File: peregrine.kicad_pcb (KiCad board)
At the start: 4 copper layers, 113.2 x 20.4 mm, 52 parts, among them J1 Barrel_Jack, J2 Ext., J3 Ext., J4 50Ω, SW1 SW_SPDT, SW2 SW_SPDT, U1 MIC5365-3.3YD5, U2 MIC5365-3.3YD5, U3 4020, U4 TS5A3159ADBVR, U5 74AUC1G86, U6 74AUC2G34, X1 ASV-16MHz

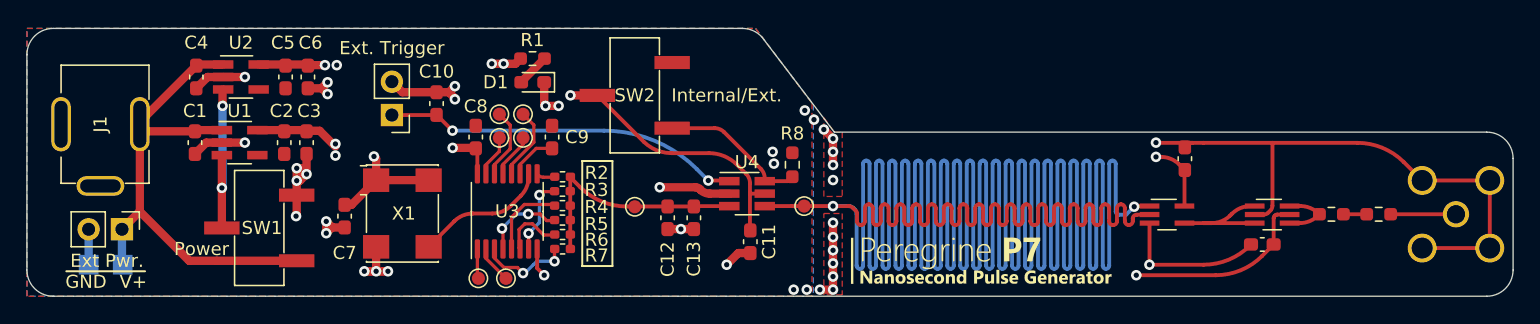
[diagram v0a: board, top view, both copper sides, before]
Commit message: this concerns me
i feel like this is not going to be pretty. might need to simulate more
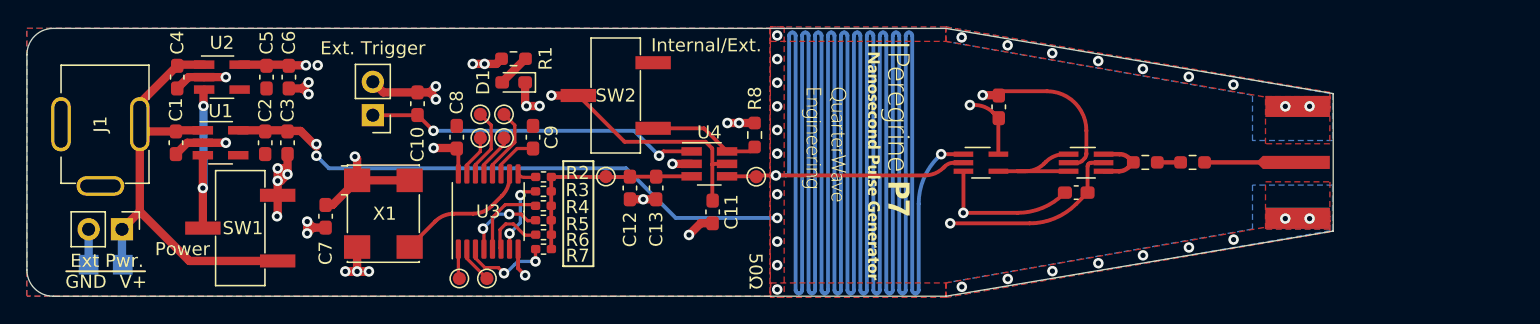
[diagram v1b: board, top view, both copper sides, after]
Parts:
- removed the G*** at (161.8, 104.7)
- added G***: LOGO, QuarterWave:logoWithText12mmPartialMask, F.Cu at (153.7, 101.7)
- J4: footprint SMA_RightAngle:SMA-RightAngle -> CONSMA020:LINX_CONSMA020.062-G
- moved R10 14.7 mm to (181.8, 104.6)
- moved R9 14.7 mm to (178.2, 104.6)
- moved C14 14.7 mm to (167.0, 100.4)
- moved C15 14.7 mm to (172.9, 106.9)
- moved U5 14.7 mm to (165.7, 104.6)
- moved U6 14.7 mm to (173.7, 104.6)
- moved G*** 10.4 mm to (158.6, 104.6), turned to -90 degrees
- moved J4 10.4 mm to (192.2, 104.6), turned to 90 degrees
- moved TP3 4.28 mm to (148.6, 105.7)
- moved C12 3.66 mm to (138.9, 106.6)
- moved C13 3.66 mm to (140.9, 106.6)
- moved C11 3.66 mm to (145.2, 108.4)
- moved R8 3.66 mm to (148.4, 102.5)
- moved U4 3.66 mm to (145.0, 104.7)
- moved TP4 3.18 mm to (137.1, 105.7)
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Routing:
- net GND: track 119.1 -> 72.2 mm, vias 40 -> 53
- net VCC: track 127.6 -> 134.0 mm
- net Trig: track 420.2 -> 426.0 mm
- net +VDC: track 39.6 -> 36.1 mm
- net Net-(R8-Pad1): track 11.2 -> 8.60 mm
- net FTrig: track 18.5 -> 16.4 mm
- net Net-(J4-Pad1): track 4.97 -> 6.74 mm
- net +3V3: track 75.8 -> 74.1 mm
- net Net-(C10-Pad1): track 27.3 -> 25.8 mm
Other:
- board size 113.2 x 20.4 mm -> 99.5 x 20.4 mm

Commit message: redesign
why yes i redesigned half of the entire board
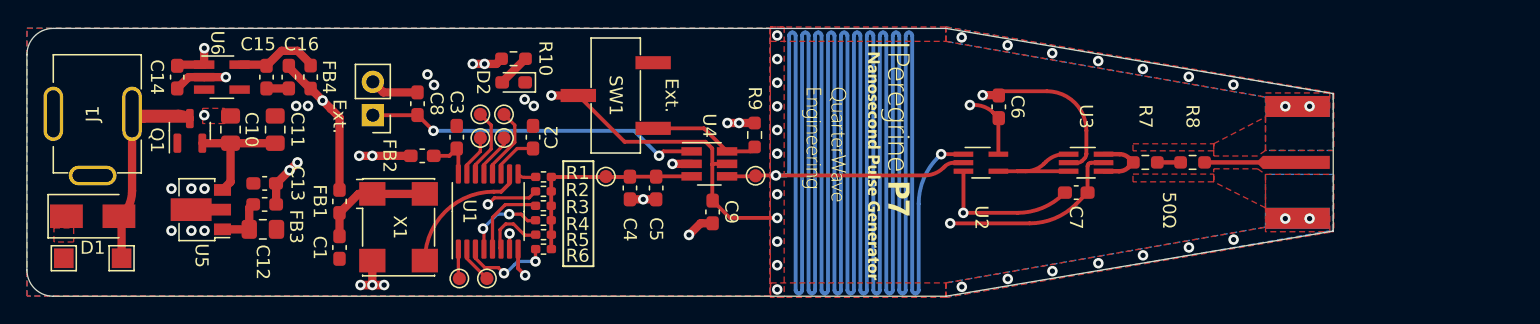
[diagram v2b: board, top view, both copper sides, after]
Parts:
- removed the C1 at (104.3, 103.1)
- removed the C2 at (111.2, 103.1)
- removed the J2 at (100.2, 109.7)
- removed the SW1 at (109.2, 109.6)
- removed the TP1 at (100.3, 112.4)
- removed the TP2 at (97.7, 112.4)
- removed the U1 at (107.8, 103.1)
- added C10: 10μF, Capacitor_SMD:C_0805_2012Metric_Pad1.18x1.45mm_HandSolder, F.Cu at (108.5, 102.1)
- added C11: 330nF, Capacitor_SMD:C_0805_2012Metric_Pad1.18x1.45mm_HandSolder, F.Cu at (111.9, 102.1)
- added C12: 10μF, Capacitor_SMD:C_0805_2012Metric_Pad1.18x1.45mm_HandSolder, F.Cu at (111.0, 109.7)
- added D1: SMAJ30A, Diode_SMD:D_SMA, F.Cu at (98.0, 108.7)
- added FB1: FerriteBead_Small, Inductor_SMD:L_0603_1608Metric_Pad1.05x0.95mm_HandSolder, F.Cu at (116.8, 107.6)
- added FB2: FerriteBead_Small, Inductor_SMD:L_0603_1608Metric_Pad1.05x0.95mm_HandSolder, F.Cu at (123.1, 104.1)
- added FB3: FerriteBead_Small, Inductor_SMD:L_0603_1608Metric_Pad1.05x0.95mm_HandSolder, F.Cu at (111.1, 107.8)
- added FB4: FerriteBead_Small, Inductor_SMD:L_0603_1608Metric_Pad1.05x0.95mm_HandSolder, F.Cu at (114.6, 98.1)
- added Q1: BSS84, Package_TO_SOT_SMD:SOT-23, F.Cu at (105.4, 102.2)
- added REF**: ESD-Logo_13.2x12mm_SilkScreen, Symbol:ESD-Logo_13.2x12mm_SilkScreen, B.Cu at (168.0, 104.6)
- added TP10: GND, TestPoint:TestPoint_Pad_1.5x1.5mm, F.Cu at (95.8, 111.9)
- added TP9: V+, TestPoint:TestPoint_Pad_1.5x1.5mm, F.Cu at (100.2, 111.9)
- added U5: L78L05_SOT89, Package_TO_SOT_SMD:SOT-89-3, F.Cu at (106.2, 108.2)
- moved REF** 15.9 mm to (140.6, 104.6), turned to 90 degrees
- moved C13 3.55 mm to (111.1, 106.2), turned to 180 degrees
- moved C1 2.60 mm to (116.8, 111.1)
- moved X1 1.55 mm to (121.3, 109.6)
- moved J1 0.99 mm to (95.0, 100.9)
- moved TP7 0.09 mm to (148.5, 105.6)
- renumbered C7 to C1, C3 to C13, C4 to C14, C5 to C15, C6 to C16, C9 to C2, C8 to C3, C12 to C4, C13 to C5, C14 to C6, C15 to C7, C10 to C8, C11 to C9, D1 to D2, J3 to J2, J4 to J3, R2 to R1, R1 to R10, R3 to R2, R4 to R3, R5 to R4, R6 to R5, R7 to R6, R9 to R7, R10 to R8, R8 to R9, SW2 to SW1, TP5 to TP1, TP6 to TP2, TP7 to TP3, TP8 to TP4, TP9 to TP5, TP10 to TP6, TP3 to TP7, TP4 to TP8, U3 to U1, U5 to U2, U6 to U3, U2 to U6
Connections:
- net FTrig renamed /peregrineSelector/FTrig
- net Net-(C10-Pad1) renamed /peregrineSelector/ExtTrig
- net Net-(J4-Pad1) renamed /peregrinePulser/Output
- net Trig renamed /peregrinePulser/Trig
- C1 pad 1: +3V3 -> Net-(C1-Pad1)
- C13 pad 1: VCC -> +5V
- C14 pad 1: +VDC -> +5V
- C15 pad 1: +3V3 -> Net-(C15-Pad1)
- C3 pad 1: +3V3 -> Net-(C3-Pad1)
- C6 pad 2: VCC -> +3V3
- C7 pad 1: VCC -> +3V3
- U1 pad 16: +3V3 -> Net-(C3-Pad1)
- U2 pad 5: VCC -> +3V3
- U3 pad 5: VCC -> +3V3
- U6 pad 1: +VDC -> +5V
- U6 pad 5: +3V3 -> Net-(C15-Pad1)
- X1 pad 1: +3V3 -> Net-(C1-Pad1)
- X1 pad 4: +3V3 -> Net-(C1-Pad1)
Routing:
- net VCC: track 134.0 -> 0.00 mm, vias 5 -> 0
- net +3V3: track 74.1 -> 157.8 mm
- net +5V: track 0.00 -> 43.4 mm, vias 0 -> 5
- net GND: track 72.2 -> 49.3 mm
- net +VDC: track 36.1 -> 20.0 mm
- net PWR: track 13.1 -> 0.00 mm, vias 2 -> 0
- net Net-(C10-Pad1): track 0.00 -> 9.37 mm
- net Net-(C1-Pad1): track 0.00 -> 8.87 mm
- net Net-(C15-Pad1): track 0.00 -> 6.44 mm
- net Net-(C12-Pad1): track 0.00 -> 4.10 mm
- net Net-(C3-Pad1): track 0.00 -> 3.95 mm
- net Net-(R2-Pad2): track 5.71 -> 8.13 mm
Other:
- board text added: "6/18/22"
- board text added: "Ext."
- board text added: "Revision 3"
- board text removed: "Ext Pwr."
- board text removed: "Ext. Trigger"
- board text removed: "GND"
- board text removed: "Internal/Ext."
- board text removed: "Power"
- board text removed: "V+"
